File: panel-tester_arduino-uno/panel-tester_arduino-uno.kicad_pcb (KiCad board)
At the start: 2 copper layers, 66 x 54 mm, 2 parts, among them J1 Conn_01x15_Female

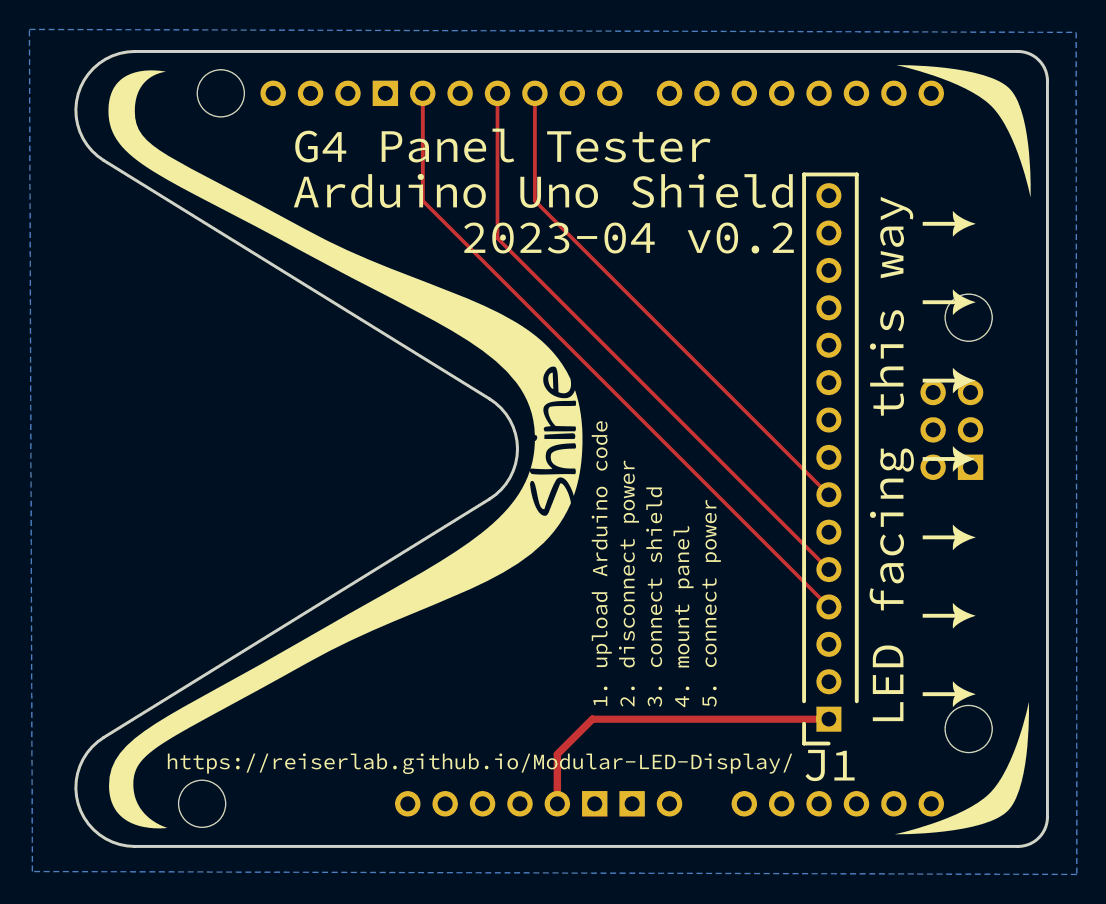
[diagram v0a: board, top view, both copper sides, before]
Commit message: make tester ready for order
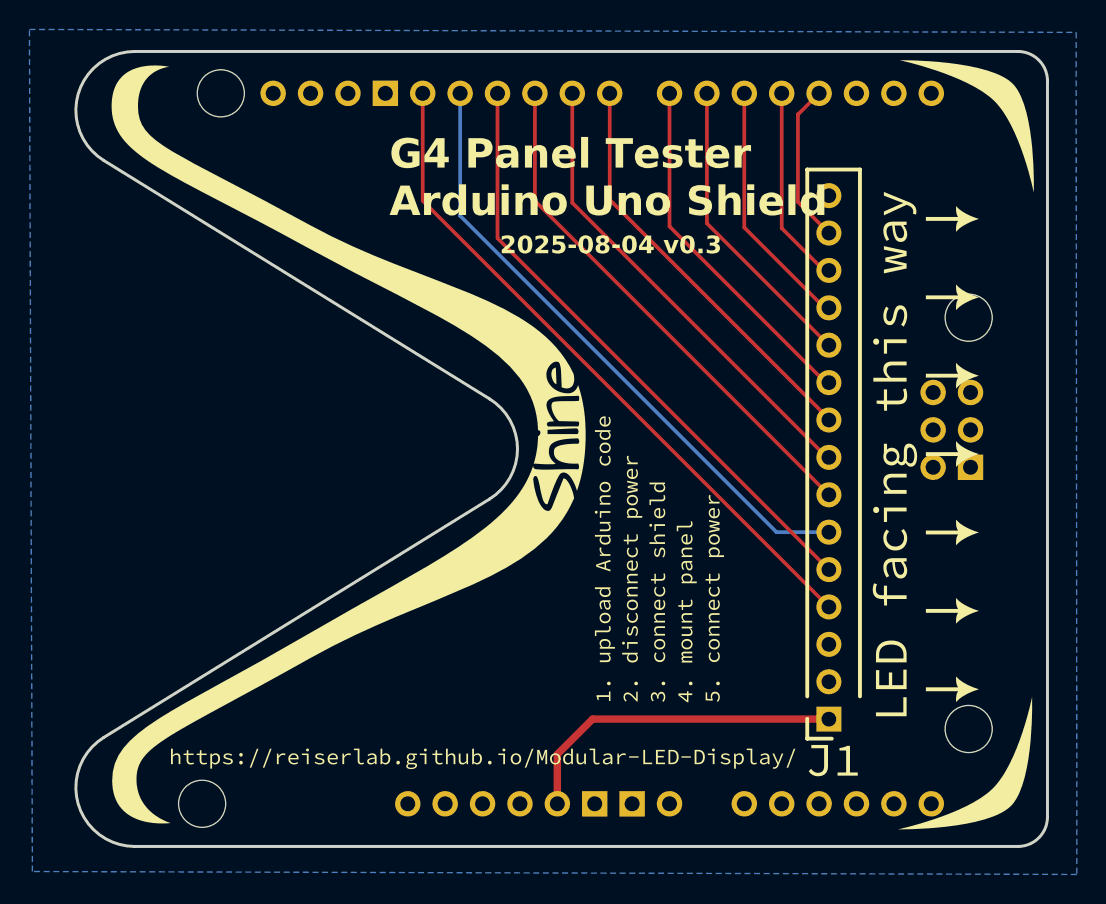
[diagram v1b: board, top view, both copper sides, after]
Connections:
- J1 pad 10: unconnected-(J1-Pad10) -> /CS3
- J1 pad 11: unconnected-(J1-Pad11) -> /CS4
- J1 pad 12: unconnected-(J1-Pad12) -> /CS5
- J1 pad 13: unconnected-(J1-Pad13) -> /CS6
- J1 pad 14: unconnected-(J1-Pad14) -> /CS7
- J1 pad 6: unconnected-(J1-Pad6) -> /CIPO
- J1 pad 7: /CS1 -> /CS0
- J1 pad 8: unconnected-(J1-Pad8) -> /CS1
- J1 pad 9: unconnected-(J1-Pad9) -> /CS2
- XA1 pad D10: /CS1 -> /CS0
- XA1 pad D12: unconnected-(XA1-PadD12) -> /CIPO
- XA1 pad D3: unconnected-(XA1-PadD3) -> /CS7
- XA1 pad D4: unconnected-(XA1-PadD4) -> /CS6
- XA1 pad D5: unconnected-(XA1-PadD5) -> /CS5
- XA1 pad D6: unconnected-(XA1-PadD6) -> /CS4
- XA1 pad D7: unconnected-(XA1-PadD7) -> /CS3
- XA1 pad D8: unconnected-(XA1-PadD8) -> /CS2
- XA1 pad D9: unconnected-(XA1-PadD9) -> /CS1
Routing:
- net /CIPO: track 0.00 -> 42.3 mm
- net /CS0: track 0.00 -> 35.5 mm
- net /CS2: track 0.00 -> 28.4 mm
- net /CS3: track 0.00 -> 24.3 mm
- net /CS4: track 0.00 -> 20.5 mm
- net /CS5: track 0.00 -> 17.1 mm
- net /CS6: track 0.00 -> 13.6 mm
- net /CS7: track 0.00 -> 11.0 mm
- net /CS1: track 35.5 -> 32.0 mm
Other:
- board text added: "${ISSUE_DATE} ${REVISION}"
- board text added: "${TITLE} Arduino Uno Shield"
